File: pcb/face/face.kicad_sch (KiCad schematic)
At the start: 26 parts, among them J1 26 pin IDC, J2 Phoenix MSTB, U1 K155ID1, U2 K155ID1, U3 K155ID1, U4 K155ID1

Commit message: Final Rev B
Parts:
- J1, J2, NX1, NX2, NX3, NX4, NX5, NX6, U1, U2, U3, U4: now left out of the parts list
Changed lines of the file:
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@@
 		(unit 1)
 		(exclude_from_sim no)
-		(in_bom yes)
+		(in_bom no)
 		(on_board yes)
 		(dnp no)
@@
 		(unit 1)
 		(exclude_from_sim no)
-		(in_bom yes)
+		(in_bom no)
 		(on_board yes)
 		(dnp no)
@@
 			)
 		)
+		(property "LCSC" ""
+			(at 46.99 91.44 0)
+			(effects
+				(font
+					(size 1.27 1.27)
+				)
+				(hide yes)
+			)
+		)
 		(pin "3"
 		)
@@
 		(unit 1)
 		(exclude_from_sim no)
-		(in_bom yes)
+		(in_bom no)
 		(on_board yes)
 		(dnp no)
@@
 		(unit 1)
 		(exclude_from_sim no)
-		(in_bom yes)
+		(in_bom no)
 		(on_board yes)
 		(dnp no)
@@
 		(unit 1)
 		(exclude_from_sim no)
-		(in_bom yes)
+		(in_bom no)
 		(on_board yes)
 		(dnp no)
@@
 		(unit 1)
 		(exclude_from_sim no)
-		(in_bom yes)
+		(in_bom no)
 		(on_board yes)
 		(dnp no)
@@
 		(unit 1)
 		(exclude_from_sim no)
-		(in_bom yes)
+		(in_bom no)
 		(on_board yes)
 		(dnp no)
@@
 		(unit 1)
 		(exclude_from_sim no)
-		(in_bom yes)
+		(in_bom no)
 		(on_board yes)
 		(dnp no)
@@
 		(unit 1)
 		(exclude_from_sim no)
-		(in_bom yes)
+		(in_bom no)
 		(on_board yes)
 		(dnp no)
@@
 		(unit 1)
 		(exclude_from_sim no)
-		(in_bom yes)
+		(in_bom no)
 		(on_board yes)
 		(dnp no)
@@
 			)
 		)
+		(property "LCSC" ""
+			(at 129.54 90.17 0)
+			(effects
+				(font
+					(size 1.27 1.27)
+				)
+				(hide yes)
+			)
+		)
 		(pin "3"
 		)
@@
 		(unit 1)
 		(exclude_from_sim no)
-		(in_bom yes)
+		(in_bom no)
 		(on_board yes)
 		(dnp no)
@@
 			)
 		)
+		(property "LCSC" ""
+			(at 129.54 40.64 0)
+			(effects
+				(font
+					(size 1.27 1.27)
+				)
+				(hide yes)
+			)
+		)
 		(pin "3"
 		)
@@
 		(unit 1)
 		(exclude_from_sim no)
-		(in_bom yes)
+		(in_bom no)
 		(on_board yes)
 		(dnp no)

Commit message: HV converter Rev C redesign around LM5156
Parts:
- C1, C2, C3, C4: footprint nixie_clock:C_Rect_L5.1mm_W3.2mm_P2.54mm_Goldmax -> 0_nixie_clock:C_Rect_L5.1mm_W3.2mm_P2.54mm_Goldmax
- NX1, NX4: footprint nixie_clock:IN-6 -> 0_nixie_clock:IN-6; symbol nixie_clock:IN-6 -> 0_nixie_clock:IN-6
- NX2, NX3, NX5, NX6: footprint nixie_clock:IN-12-DSUB -> 0_nixie_clock:IN-12-DSUB; symbol nixie_clock:IN-12B -> 0_nixie_clock:IN-12B
- U1, U2, U3, U4: footprint nixie_clock:DIP16 -> 0_nixie_clock:DIP16; symbol nixie_clock:K155ID1 -> 0_nixie_clock:K155ID1
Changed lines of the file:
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@@
 			)
 		)
-		(property "Footprint" "nixie_clock:C_Rect_L5.1mm_W3.2mm_P2.54mm_Goldmax"
+		(property "Footprint" "0_nixie_clock:C_Rect_L5.1mm_W3.2mm_P2.54mm_Goldmax"
 			(at 107.6452 85.09 0)
 			(effects
@@
 	)
 	(symbol
-		(lib_id "nixie_clock:K155ID1")
+		(lib_id "0_nixie_clock:K155ID1")
 		(at 46.99 41.91 0)
 		(unit 1)
@@
 			)
 		)
-		(property "Footprint" "nixie_clock:DIP16"
+		(property "Footprint" "0_nixie_clock:DIP16"
 			(at 47.752 38.1 0)
 			(effects
@@
 	)
 	(symbol
-		(lib_id "nixie_clock:K155ID1")
+		(lib_id "0_nixie_clock:K155ID1")
 		(at 46.99 91.44 0)
 		(unit 1)
@@
 			)
 		)
-		(property "Footprint" "nixie_clock:DIP16"
+		(property "Footprint" "0_nixie_clock:DIP16"
 			(at 47.752 87.63 0)
 			(effects
@@
 			)
 		)
-		(property "Footprint" "nixie_clock:C_Rect_L5.1mm_W3.2mm_P2.54mm_Goldmax"
+		(property "Footprint" "0_nixie_clock:C_Rect_L5.1mm_W3.2mm_P2.54mm_Goldmax"
 			(at 107.6452 35.56 0)
 			(effects
@@
 	)
 	(symbol
-		(lib_id "nixie_clock:IN-6")
+		(lib_id "0_nixie_clock:IN-6")
 		(at 204.47 59.69 0)
 		(unit 1)
@@
 			)
 		)
-		(property "Footprint" "nixie_clock:IN-6"
+		(property "Footprint" "0_nixie_clock:IN-6"
 			(at 205.232 55.88 0)
 			(effects
@@
 	)
 	(symbol
-		(lib_id "nixie_clock:IN-12B")
+		(lib_id "0_nixie_clock:IN-12B")
 		(at 157.48 92.71 0)
 		(unit 1)
@@
 			)
 		)
-		(property "Footprint" "nixie_clock:IN-12-DSUB"
+		(property "Footprint" "0_nixie_clock:IN-12-DSUB"
 			(at 158.242 88.9 0)
 			(effects
@@
 	)
 	(symbol
-		(lib_id "nixie_clock:IN-12B")
+		(lib_id "0_nixie_clock:IN-12B")
 		(at 74.93 44.45 0)
 		(unit 1)
@@
 			)
 		)
-		(property "Footprint" "nixie_clock:IN-12-DSUB"
+		(property "Footprint" "0_nixie_clock:IN-12-DSUB"
 			(at 75.692 40.64 0)
 			(effects
@@
 	)
 	(symbol
-		(lib_id "nixie_clock:IN-12B")
+		(lib_id "0_nixie_clock:IN-12B")
 		(at 157.48 43.18 0)
 		(unit 1)
@@
 			)
 		)
-		(property "Footprint" "nixie_clock:IN-12-DSUB"
+		(property "Footprint" "0_nixie_clock:IN-12-DSUB"
 			(at 158.242 39.37 0)
 			(effects
@@
 	)
 	(symbol
-		(lib_id "nixie_clock:IN-12B")
+		(lib_id "0_nixie_clock:IN-12B")
 		(at 74.93 93.98 0)
 		(unit 1)
@@
 			)
 		)
-		(property "Footprint" "nixie_clock:IN-12-DSUB"
+		(property "Footprint" "0_nixie_clock:IN-12-DSUB"
 			(at 75.692 90.17 0)
 			(effects
@@
 			)
 		)
-		(property "Footprint" "nixie_clock:C_Rect_L5.1mm_W3.2mm_P2.54mm_Goldmax"
+		(property "Footprint" "0_nixie_clock:C_Rect_L5.1mm_W3.2mm_P2.54mm_Goldmax"
 			(at 25.0952 86.36 0)
 			(effects
@@
 			)
 		)
-		(property "Footprint" "nixie_clock:C_Rect_L5.1mm_W3.2mm_P2.54mm_Goldmax"
+		(property "Footprint" "0_nixie_clock:C_Rect_L5.1mm_W3.2mm_P2.54mm_Goldmax"
 			(at 25.0952 36.83 0)
 			(effects
@@
 	)
 	(symbol
-		(lib_id "nixie_clock:K155ID1")
+		(lib_id "0_nixie_clock:K155ID1")
 		(at 129.54 90.17 0)
 		(unit 1)
@@
 			)
 		)
-		(property "Footprint" "nixie_clock:DIP16"
+		(property "Footprint" "0_nixie_clock:DIP16"
 			(at 130.302 86.36 0)
 			(effects
@@
 	)
 	(symbol
-		(lib_id "nixie_clock:K155ID1")
+		(lib_id "0_nixie_clock:K155ID1")
 		(at 129.54 40.64 0)
 		(unit 1)
@@
 			)
 		)
-		(property "Footprint" "nixie_clock:DIP16"
+		(property "Footprint" "0_nixie_clock:DIP16"
 			(at 130.302 36.83 0)
 			(effects
@@
 	)
 	(symbol
-		(lib_id "nixie_clock:IN-6")
+		(lib_id "0_nixie_clock:IN-6")
 		(at 204.47 36.83 0)
 		(unit 1)
@@
 			)
 		)
-		(property "Footprint" "nixie_clock:IN-6"
+		(property "Footprint" "0_nixie_clock:IN-6"
 			(at 205.232 33.02 0)
 			(effects

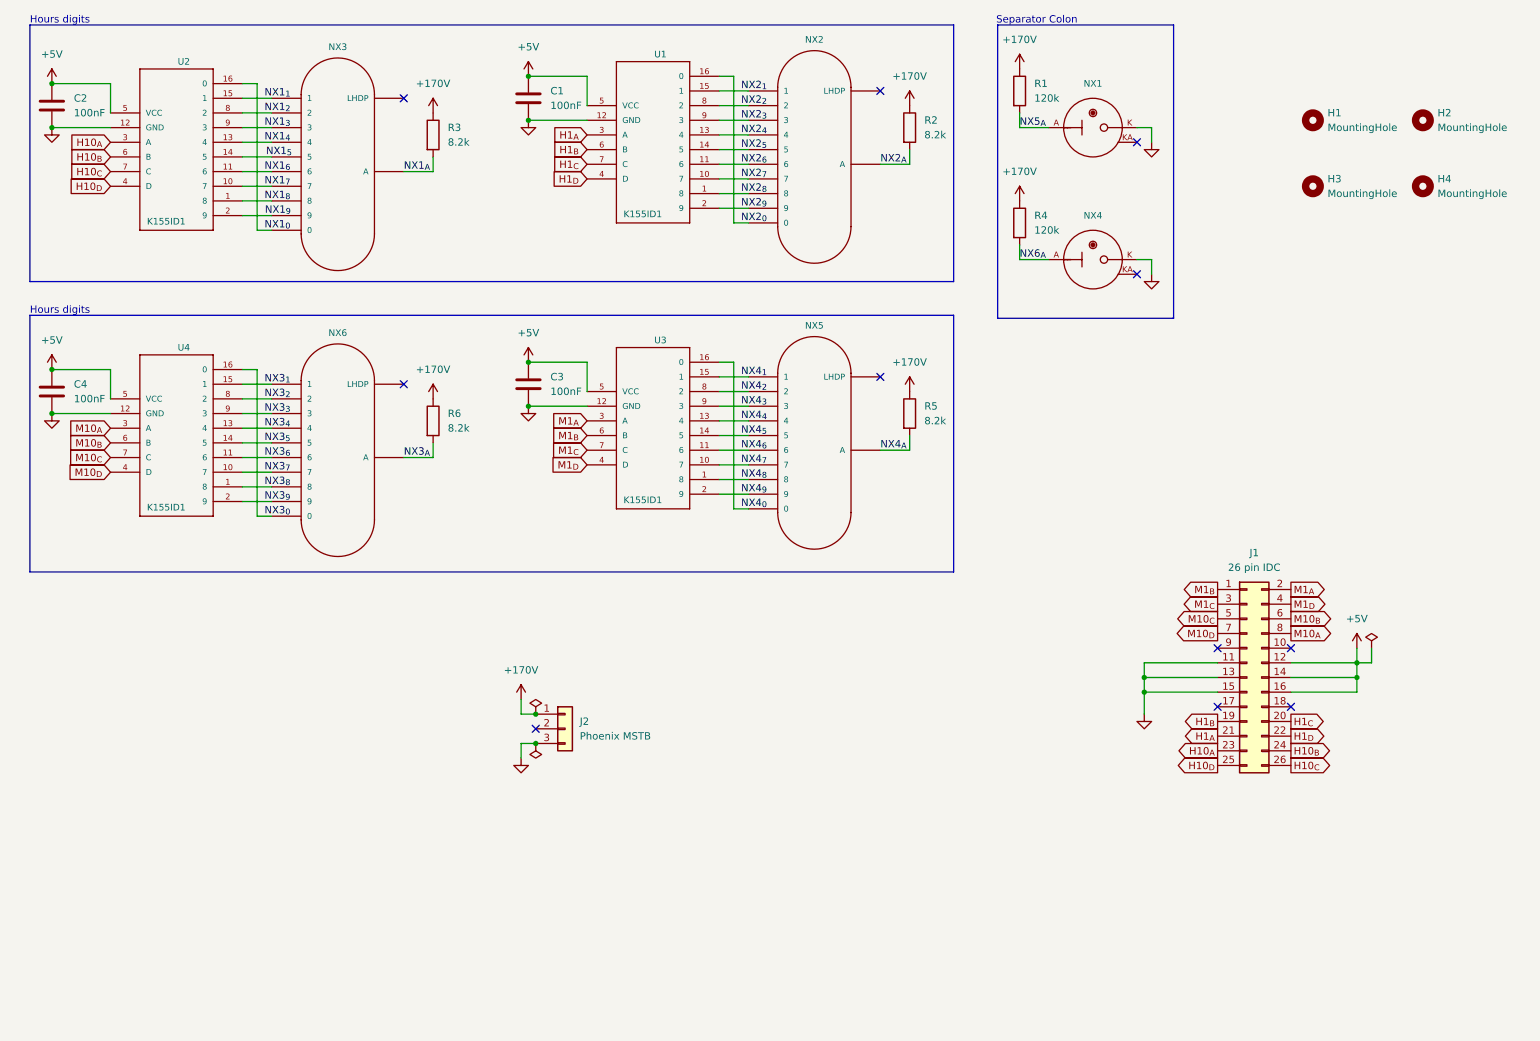
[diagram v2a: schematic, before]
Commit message: Clock Face Rev C
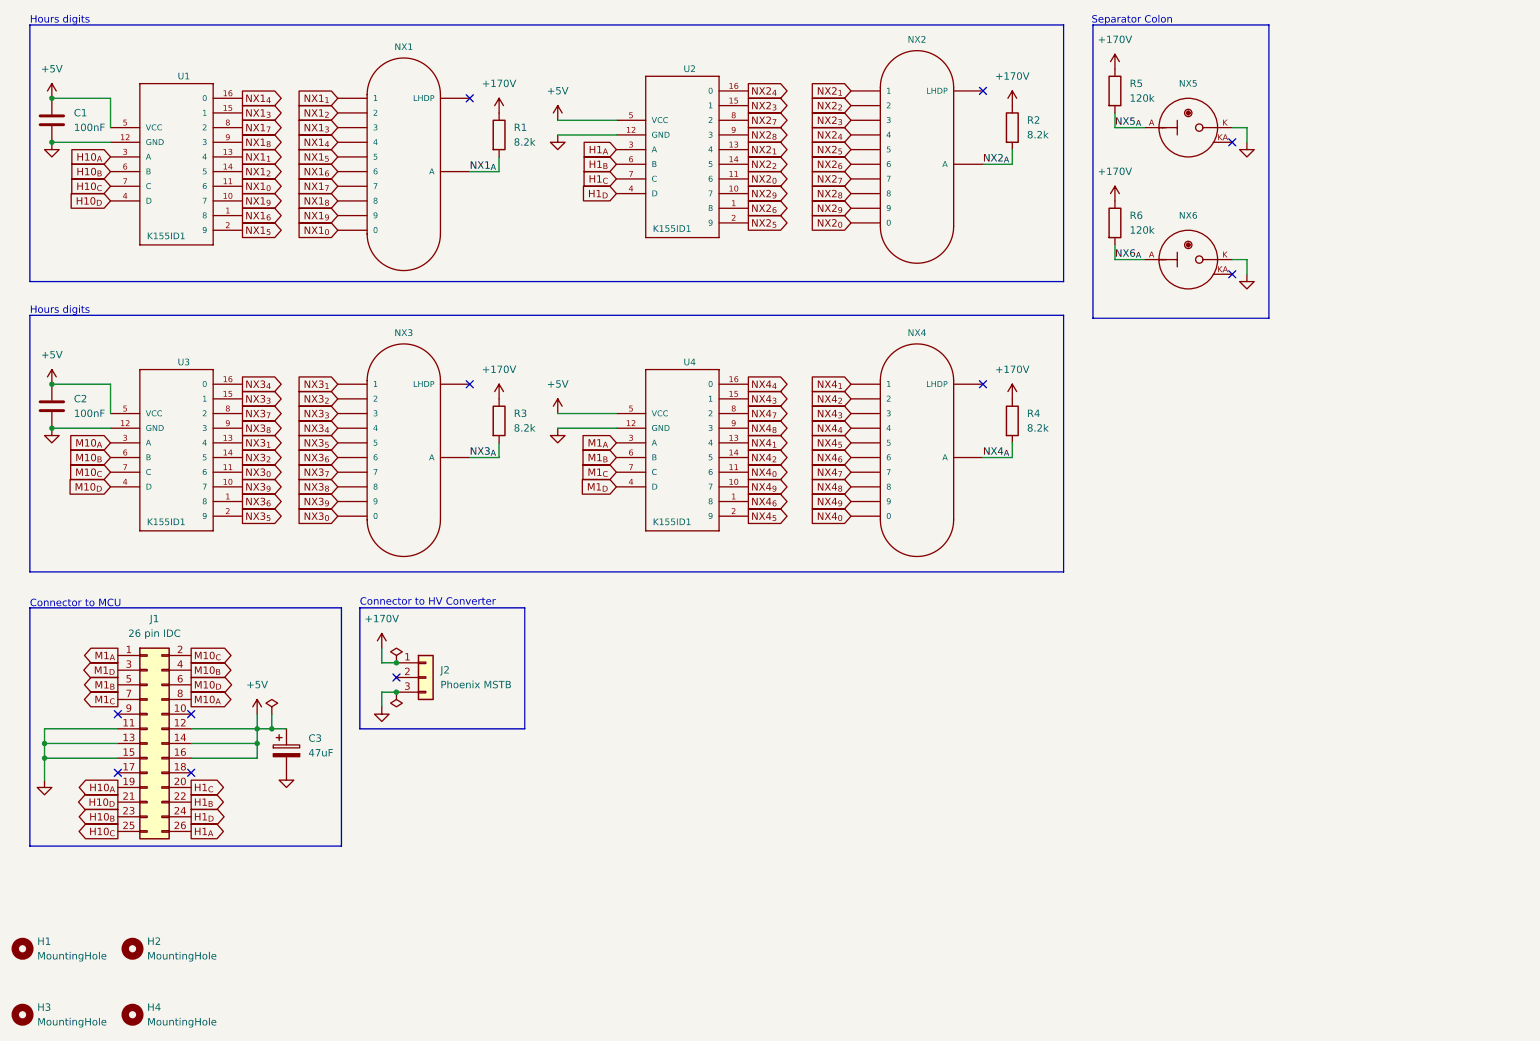
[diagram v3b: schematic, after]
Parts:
- removed C1, C3: 100nF, 0_nixie_clock:C_Rect_L5.1mm_W3.2mm_P2.54mm_Goldmax, symbol Device:C
- added C3: 47uF, 0_nixie_clock:CP_Radial_D6.3mm_P2.50mm, symbol Device:C_Polarized
- renumbered C2 to C1, C4 to C2, NX3 to NX1, NX6 to NX3, NX5 to NX4, NX1 to NX5, NX4 to NX6, R3 to R1, R6 to R3, R5 to R4, R1 to R5, R4 to R6, U2 to U1, U1 to U2, U4 to U3, U3 to U4
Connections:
- net +5V: now also C3.1
- net GND: now also C3.2
- net H10_{A}: now also J1.19 (Pin_19); no longer J1.23 (Pin_23)
- net H10_{B}: now also J1.23 (Pin_23); no longer J1.24 (Pin_24)
- net H10_{C}: now also J1.25 (Pin_25); no longer J1.26 (Pin_26)
- net H10_{D}: now also J1.21 (Pin_21); no longer J1.25 (Pin_25)
- net H1_{A}: now also J1.26 (Pin_26); no longer J1.21 (Pin_21)
- net H1_{B}: now also J1.22 (Pin_22); no longer J1.19 (Pin_19)
- net H1_{D}: now also J1.24 (Pin_24); no longer J1.22 (Pin_22)
- net M10_{B}: now also J1.4 (Pin_4); no longer J1.6 (Pin_6)
- net M10_{C}: now also J1.2 (Pin_2); no longer J1.5 (Pin_5)
- net M10_{D}: now also J1.6 (Pin_6); no longer J1.7 (Pin_7)
- net M1_{A}: now also J1.1 (Pin_1); no longer J1.2 (Pin_2)
- net M1_{B}: now also J1.5 (Pin_5); no longer J1.1 (Pin_1)
- net M1_{C}: now also J1.7 (Pin_7); no longer J1.3 (Pin_3)
- net M1_{D}: now also J1.3 (Pin_3); no longer J1.4 (Pin_4)
- net NX1_{0}: now also U1.11 (6); no longer U1.16 (0)
- net NX1_{1}: now also U1.13 (4); no longer U1.15 (1)
- net NX1_{2}: now also U1.14 (5); no longer U1.8 (2)
- net NX1_{3}: now also U1.15 (1); no longer U1.9 (3)
- net NX1_{4}: now also U1.16 (0); no longer U1.13 (4)
- net NX1_{5}: now also U1.2 (9); no longer U1.14 (5)
- net NX1_{6}: now also U1.1 (8); no longer U1.11 (6)
- net NX1_{7}: now also U1.8 (2); no longer U1.10 (7)
- net NX1_{8}: now also U1.9 (3); no longer U1.1 (8)
- net NX1_{9}: now also U1.10 (7); no longer U1.2 (9)
- net NX2_{0}: now also U2.11 (6); no longer U2.16 (0)
- net NX2_{1}: now also U2.13 (4); no longer U2.15 (1)
- net NX2_{2}: now also U2.14 (5); no longer U2.8 (2)
- net NX2_{3}: now also U2.15 (1); no longer U2.9 (3)
- net NX2_{4}: now also U2.16 (0); no longer U2.13 (4)
- net NX2_{5}: now also U2.2 (9); no longer U2.14 (5)
- net NX2_{6}: now also U2.1 (8); no longer U2.11 (6)
- net NX2_{7}: now also U2.8 (2); no longer U2.10 (7)
- net NX2_{8}: now also U2.9 (3); no longer U2.1 (8)
- net NX2_{9}: now also U2.10 (7); no longer U2.2 (9)
- net NX3_{0}: now also U3.11 (6); no longer U3.16 (0)
- net NX3_{1}: now also U3.13 (4); no longer U3.15 (1)
- net NX3_{2}: now also U3.14 (5); no longer U3.8 (2)
- net NX3_{3}: now also U3.15 (1); no longer U3.9 (3)
- net NX3_{4}: now also U3.16 (0); no longer U3.13 (4)
- net NX3_{5}: now also U3.2 (9); no longer U3.14 (5)
- net NX3_{6}: now also U3.1 (8); no longer U3.11 (6)
- net NX3_{7}: now also U3.8 (2); no longer U3.10 (7)
- net NX3_{8}: now also U3.9 (3); no longer U3.1 (8)
- net NX3_{9}: now also U3.10 (7); no longer U3.2 (9)
- net NX4_{0}: now also U4.11 (6); no longer U4.16 (0)
- net NX4_{1}: now also U4.13 (4); no longer U4.15 (1)
- net NX4_{2}: now also U4.14 (5); no longer U4.8 (2)
- net NX4_{3}: now also U4.15 (1); no longer U4.9 (3)
- net NX4_{4}: now also U4.16 (0); no longer U4.13 (4)
- net NX4_{5}: now also U4.2 (9); no longer U4.14 (5)
- net NX4_{6}: now also U4.1 (8); no longer U4.11 (6)
- net NX4_{7}: now also U4.8 (2); no longer U4.10 (7)
- net NX4_{8}: now also U4.9 (3); no longer U4.1 (8)
- net NX4_{9}: now also U4.10 (7); no longer U4.2 (9)
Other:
- note added: "Connector to HV Converter"
- note added: "Connector to MCU"
- moved on the sheet: C1, C2, H1, H2, H3, H4, J1, J2, NX1, NX2, NX3, NX4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
